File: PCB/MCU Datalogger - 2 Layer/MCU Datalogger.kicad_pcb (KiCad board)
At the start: 2 copper layers, 50.7 x 30.4 mm, 29 parts, among them J1 Conn_01x04_Pin, J2 Conn_01x04_Pin, J3 Conn_01x09_Pin, J4 Conn_02x03_Odd_Even, U1 24LC1025, U2 24LC1025, U3 DS1337S+, U4 ATMEGA328P-AU, Y1 16 MHz, Y2 32.768 Khz

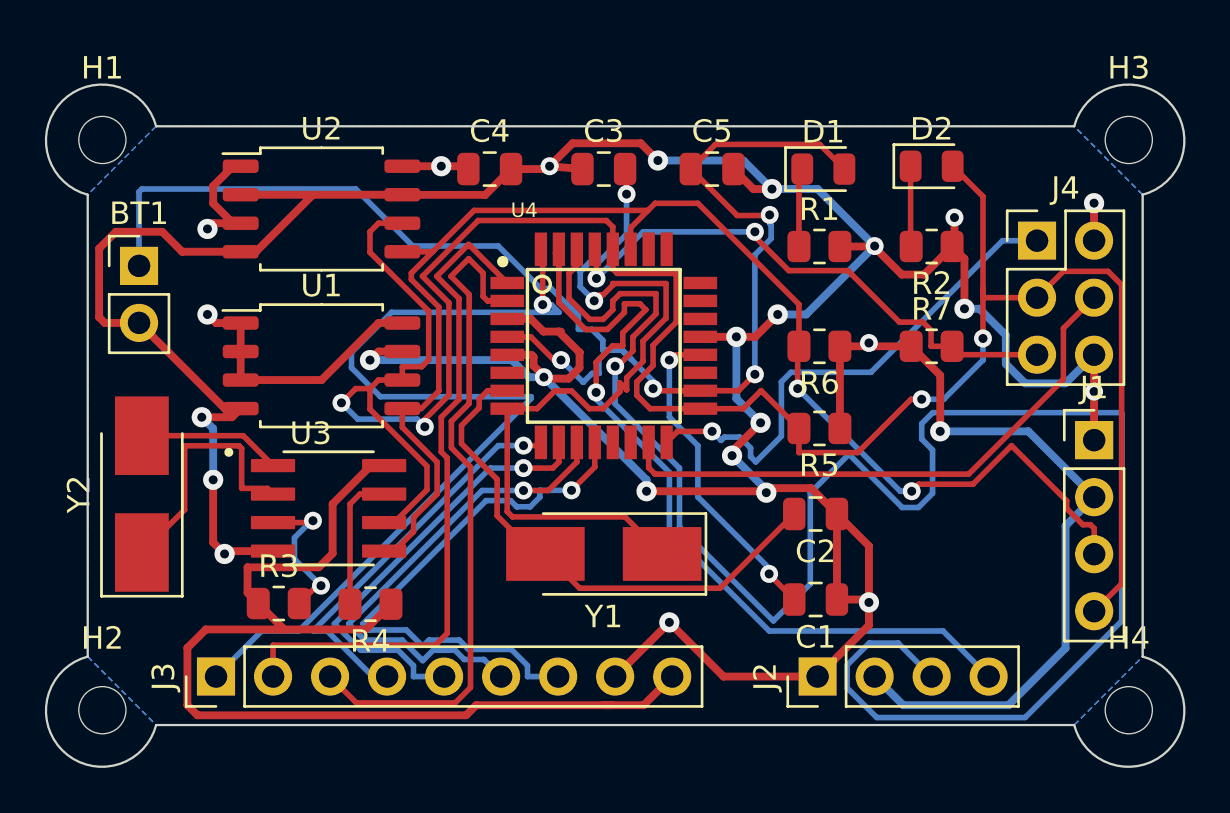
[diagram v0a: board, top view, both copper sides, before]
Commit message: Silkscreen
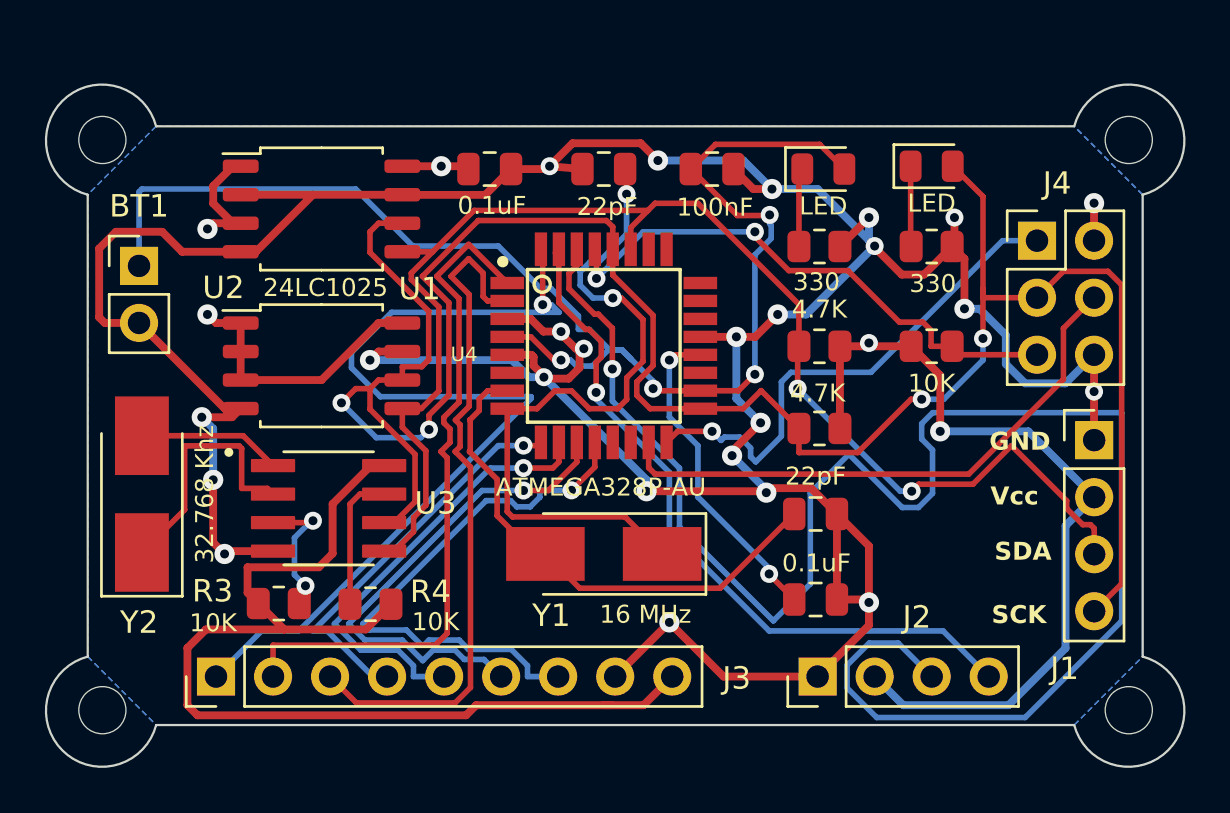
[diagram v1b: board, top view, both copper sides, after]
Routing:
- net /TX: track 37.4 -> 32.3 mm
- net /RX: track 81.5 -> 76.4 mm
- net Net-(U4-PB7): track 35.6 -> 32.3 mm
- net /SCK: track 104.9 -> 102.6 mm
- net GND: track 168.8 -> 170.8 mm, vias 20 -> 23
- net Net-(BT1-+): track 62.7 -> 61.5 mm
- net Net-(U3-~{INTA}): track 6.88 -> 6.20 mm
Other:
- board text added: "GND"
- board text added: "SCK"
- board text added: "SDA"
- board text added: "Vcc"

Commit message: Fixed violations
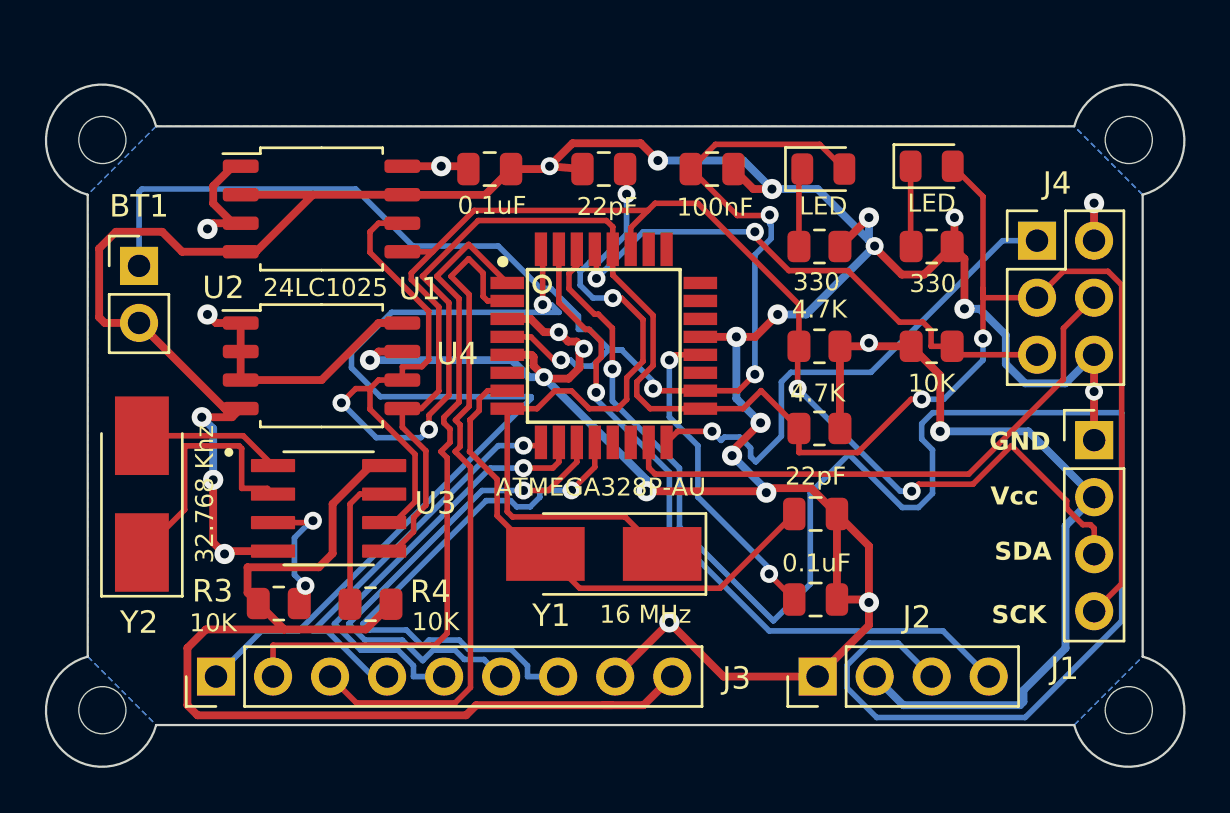
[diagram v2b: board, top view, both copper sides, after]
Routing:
- net GND: track 170.8 -> 170.1 mm
- net Net-(BT1-+): track 61.5 -> 60.9 mm
